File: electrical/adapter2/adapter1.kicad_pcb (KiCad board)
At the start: 2 copper layers, 12 x 49 mm, 7 parts, among them J2 Conn_01x08_Pin

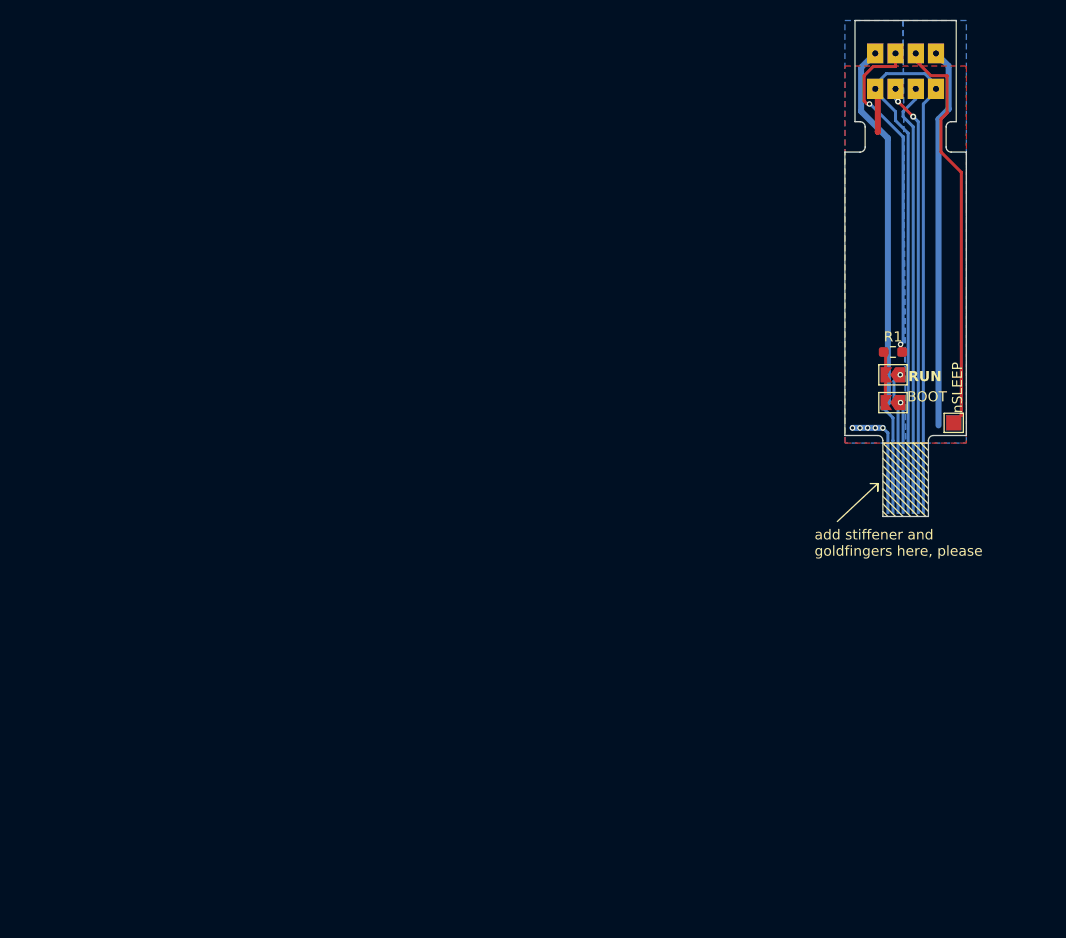
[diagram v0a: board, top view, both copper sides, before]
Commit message: start working on adapter2 PCB
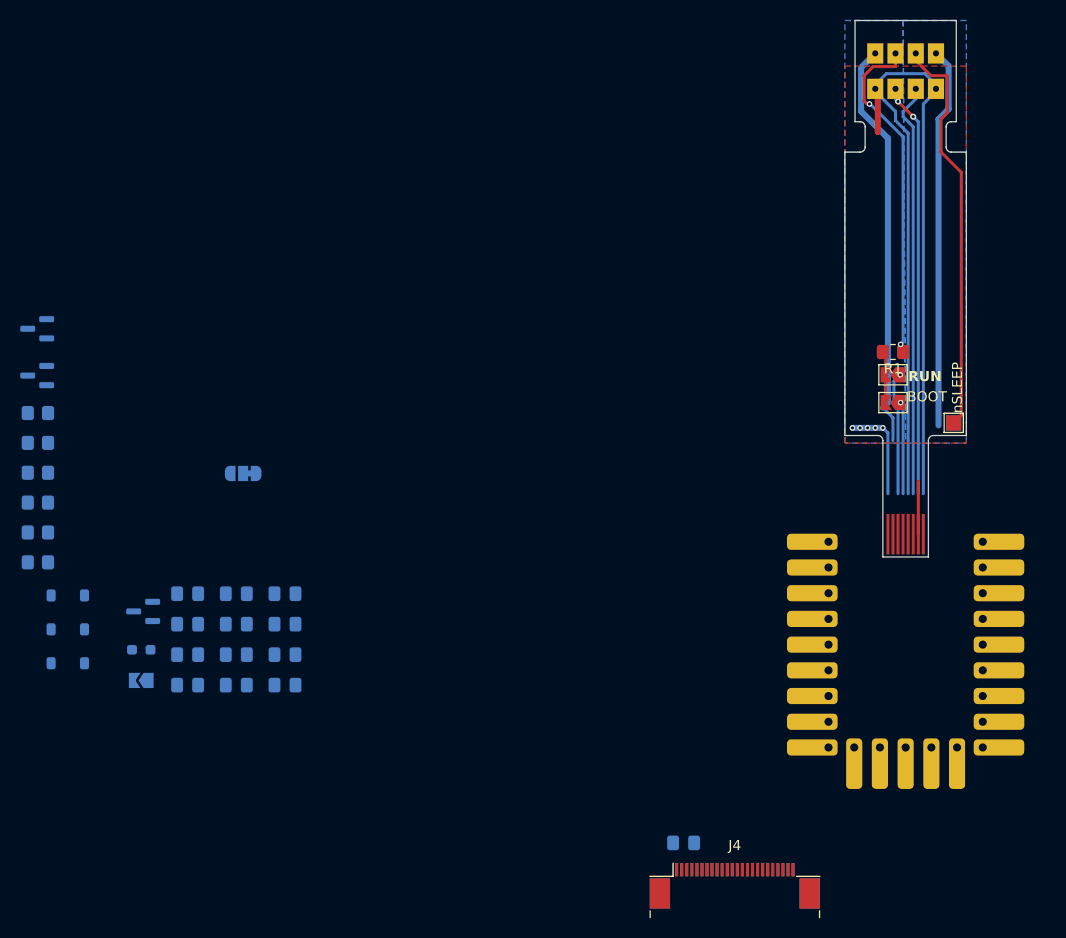
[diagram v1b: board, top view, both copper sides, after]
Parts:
- added C1: 105, Capacitor_SMD:C_0805_2012Metric_Pad1.18x1.45mm_HandSolder, B.Cu at (103.6, 121.8)
- added C10: 105, Capacitor_SMD:C_0805_2012Metric_Pad1.18x1.45mm_HandSolder, B.Cu at (54.6, 97.1)
- added C11: 105, Capacitor_SMD:C_0805_2012Metric_Pad1.18x1.45mm_HandSolder, B.Cu at (54.6, 100.1)
- added C12: 105, Capacitor_SMD:C_0805_2012Metric_Pad1.18x1.45mm_HandSolder, B.Cu at (54.6, 103.2)
- added C15: 104 !, Capacitor_SMD:C_0805_2012Metric_Pad1.18x1.45mm_HandSolder, B.Cu at (54.6, 106.2)
- added C2: 105, Capacitor_SMD:C_0805_2012Metric_Pad1.18x1.45mm_HandSolder, B.Cu at (64.2, 97.1)
- added C3: 104 !, Capacitor_SMD:C_0805_2012Metric_Pad1.18x1.45mm_HandSolder, B.Cu at (64.2, 100.1)
- added C4: 4.7uF/50V, Capacitor_SMD:C_0805_2012Metric_Pad1.18x1.45mm_HandSolder, B.Cu at (64.2, 103.2)
- added C5: 105, Capacitor_SMD:C_0805_2012Metric_Pad1.18x1.45mm_HandSolder, B.Cu at (64.2, 106.2)
- added C6: 4.7uF/50V, Capacitor_SMD:C_0805_2012Metric_Pad1.18x1.45mm_HandSolder, B.Cu at (59.4, 97.1)
- added C7: 105, Capacitor_SMD:C_0805_2012Metric_Pad1.18x1.45mm_HandSolder, B.Cu at (59.4, 100.1)
- added C8: 105, Capacitor_SMD:C_0805_2012Metric_Pad1.18x1.45mm_HandSolder, B.Cu at (59.4, 103.2)
- added C9: 105, Capacitor_SMD:C_0805_2012Metric_Pad1.18x1.45mm_HandSolder, B.Cu at (59.4, 106.2)
- added D1: MBR0530, Diode_SMD:D_SOD-123, B.Cu at (42.7, 97.3)
- added D2: MBR0530, Diode_SMD:D_SOD-123, B.Cu at (42.7, 100.7)
- added D3: MBR0530, Diode_SMD:D_SOD-123, B.Cu at (42.7, 104.0)
- added J3: 0.5 mm, 24P, Connector_FFC-FPC:Jushuo_AFC07-S24FCA-00_1x24-1MP_P0.50_Horizontal, B.Cu at (108.6, 126.0)
- added J4: 0.5 mm, 24P, Connector_FFC-FPC:Jushuo_AFC07-S24FCA-00_1x24-1MP_P0.50_Horizontal, F.Cu at (108.6, 126.0)
- added JP3: SolderJumper_3_Bridged12, Jumper:SolderJumper-3_P1.3mm_Bridged12_RoundedPad1.0x1.5mm, B.Cu at (60.0, 85.2)
- added JP4: SolderJumper_2_Open, Jumper:SolderJumper-2_P1.3mm_Open_TrianglePad1.0x1.5mm, B.Cu at (50.0, 105.7)
- added Q1: BSS138, Package_TO_SOT_SMD:SOT-23, B.Cu at (39.7, 71.0)
- added Q2: AO3401A, Package_TO_SOT_SMD:SOT-23, B.Cu at (39.7, 75.6)
- added Q3: S8050 SMD, Package_TO_SOT_SMD:SOT-23, B.Cu at (50.2, 98.9)
- added R10: DNP, Resistor_SMD:R_0603_1608Metric_Pad0.98x0.95mm_HandSolder, B.Cu at (50.0, 102.7)
- added R2: 10k, Resistor_SMD:R_0805_2012Metric_Pad1.20x1.40mm_HandSolder, B.Cu at (39.8, 79.3)
- added R3: 100k, Resistor_SMD:R_0805_2012Metric_Pad1.20x1.40mm_HandSolder, B.Cu at (39.8, 82.2)
- added R5: 10k, Resistor_SMD:R_0805_2012Metric_Pad1.20x1.40mm_HandSolder, B.Cu at (39.8, 85.2)
- added R6: 1k, Resistor_SMD:R_0805_2012Metric_Pad1.20x1.40mm_HandSolder, B.Cu at (39.8, 88.1)
- added R7: 47k, Resistor_SMD:R_0805_2012Metric_Pad1.20x1.40mm_HandSolder, B.Cu at (39.8, 91.1)
- added R8: 47k, Resistor_SMD:R_0805_2012Metric_Pad1.20x1.40mm_HandSolder, B.Cu at (39.8, 94.0)
- added U1: ~, fw16_epaper:RP2040-Tiny, B.Cu at (125.5, 102.2)
- J2: moved to F.Cu
- R1: value DNP -> 0.47R; footprint Resistor_SMD:R_0603_1608Metric_Pad0.98x0.95mm_HandSolder -> Resistor_SMD:R_0805_2012Metric_Pad1.20x1.40mm_HandSolder
- moved J2 4.00 mm to (125.5, 91.2), turned to 0 degrees
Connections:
- R1 pad 1: Net-(J1-BOARD_ID) -> GND
- R1 pad 2: GND -> Net-(Q1-S)
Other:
- board size 12 x 49 mm -> 12 x 53 mm
- board text added: "1"
- board text added: "24"
